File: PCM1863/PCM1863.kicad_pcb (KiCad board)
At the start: 2 copper layers, 76.2 x 128.5 mm, 64 parts, among them IC1 SN74AUC1G126DCKR, IC2 NCP163ASN330T1G, IC3 NCP163ASN330T1G, IC4 TXB0101DBVT, J1 Conn_02x05_Row_Letter_First, J10 Conn_01x10_Male, J4 USB_B_Micro, J8 Conn_01x10_Male, J9 Conn_01x10_Male, U1 PCM1863, Y1 ASE-24.000MHZ-ET, Y2 ASE-22.000MHZ-ET

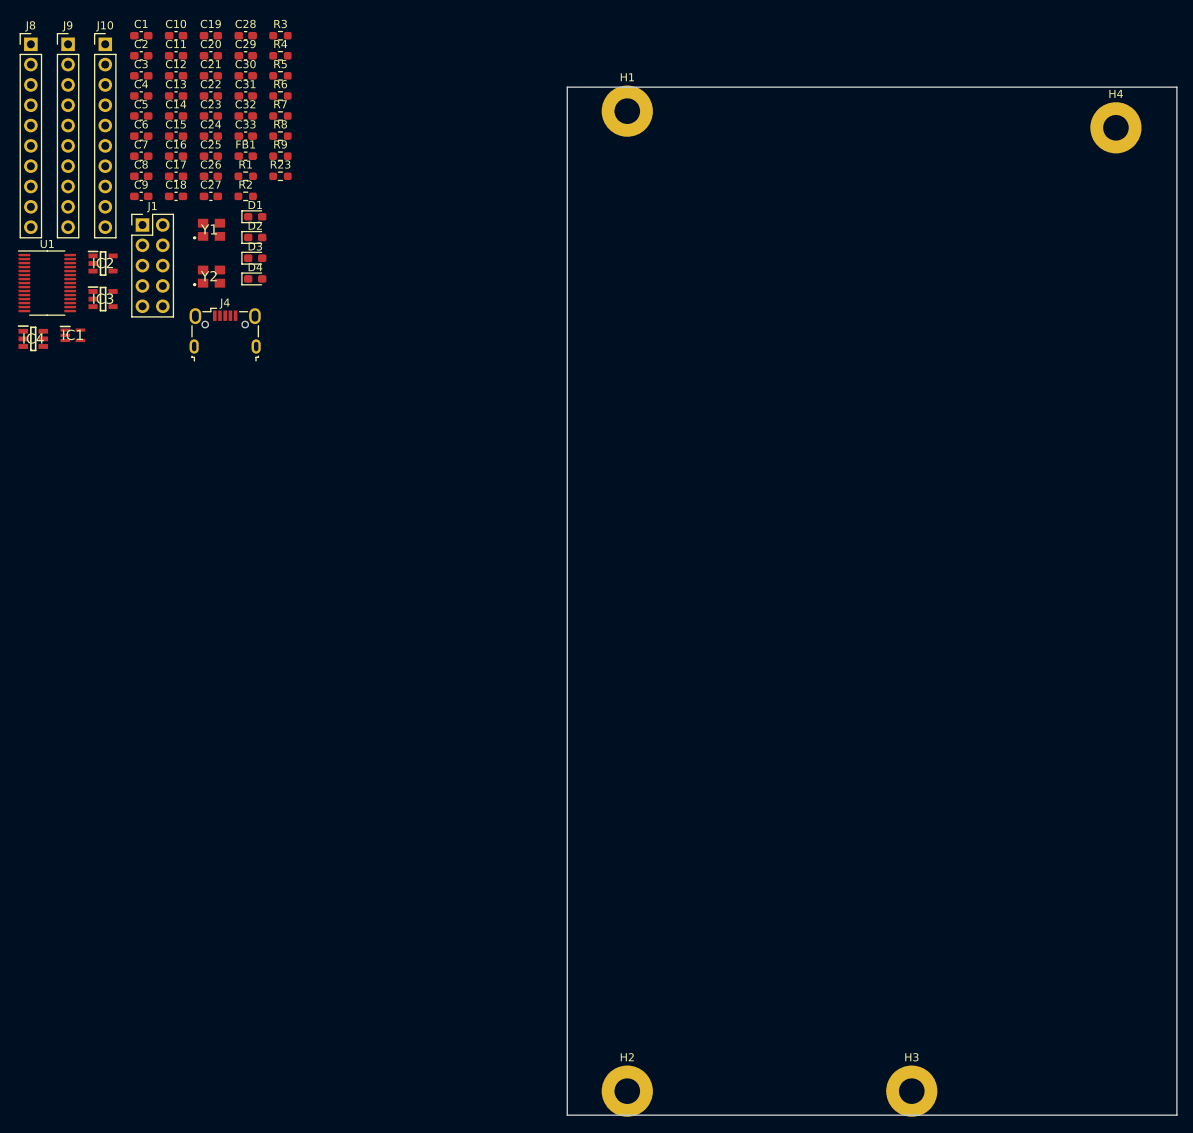
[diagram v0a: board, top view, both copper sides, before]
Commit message: Revert "Merge remote-tracking branch 'upstream/main'"
This reverts commit 91e618c32c18b3f8ce9c65181e2c7ed2aa69dacd, reversing
changes made to 5f9fe177db78953ec4a0d750e6893e90b3881885.
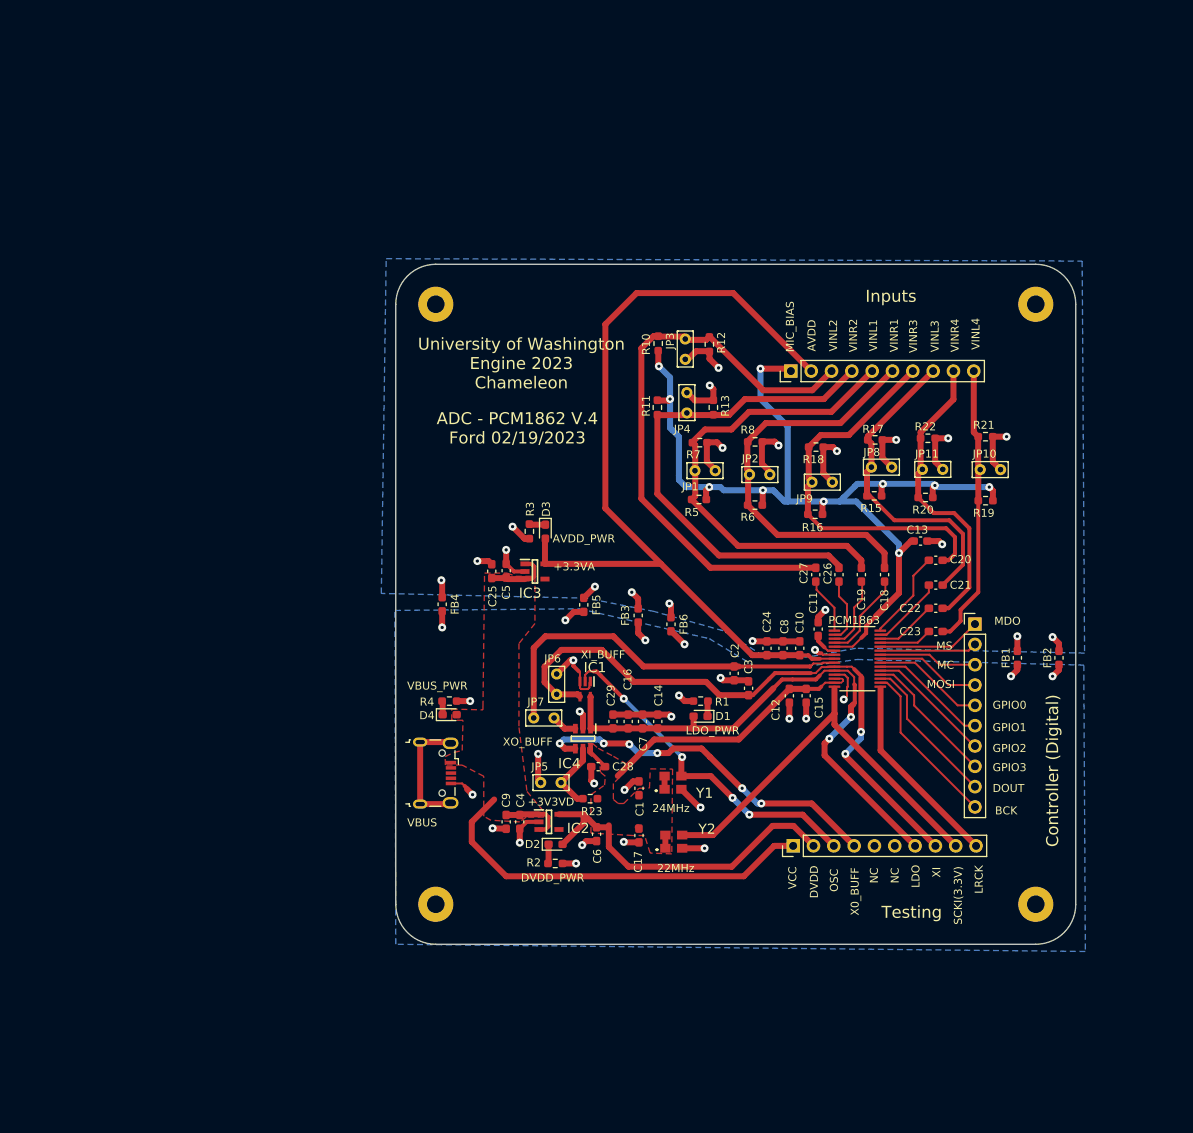
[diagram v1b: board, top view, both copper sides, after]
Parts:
- removed C30: 2.2uF, Capacitor_SMD:C_0603_1608Metric_Pad1.08x0.95mm_HandSolder
- removed C31, C33: 10uF, Capacitor_SMD:C_0603_1608Metric_Pad1.08x0.95mm_HandSolder
- removed C32: 0.01uF, Capacitor_SMD:C_0603_1608Metric_Pad1.08x0.95mm_HandSolder
- removed J10, J8, J9: Conn_01x10_Male, Connector_PinHeader_2.54mm:PinHeader_1x10_P2.54mm_Vertical
- removed R9: 4.99k, Resistor_SMD:R_0603_1608Metric_Pad0.98x0.95mm_HandSolder
- added FB2: FerriteBead, Inductor_SMD:L_0603_1608Metric_Pad1.05x0.95mm_HandSolder, F.Cu at (152.9, 94.2)
- added FB3: FerriteBead, Inductor_SMD:L_0603_1608Metric_Pad1.05x0.95mm_HandSolder, F.Cu at (100.3, 88.9)
- added FB4: FerriteBead, Inductor_SMD:L_0603_1608Metric_Pad1.05x0.95mm_HandSolder, F.Cu at (75.8, 87.5)
- added FB5: FerriteBead, Inductor_SMD:L_0603_1608Metric_Pad1.05x0.95mm_HandSolder, F.Cu at (93.5, 87.6)
- added FB6: FerriteBead, Inductor_SMD:L_0603_1608Metric_Pad1.05x0.95mm_HandSolder, F.Cu at (104.4, 90.0)
- added J2: Conn_01x10_Male, Connector_PinHeader_2.54mm:PinHeader_1x10_P2.54mm_Vertical, F.Cu at (119.4, 58.4)
- added J3: Conn_01x10_Male, Connector_PinHeader_2.54mm:PinHeader_1x10_P2.54mm_Vertical, F.Cu at (142.4, 90.0)
- added JP1: Jumper_2_Open, custom_lib:TestPoint_Bridge_Pitch2.54mm_Drill0.7mm, F.Cu at (106.2, 69.6)
- added JP10: Jumper_2_Open, custom_lib:TestPoint_Bridge_Pitch2.54mm_Drill0.7mm, F.Cu at (141.9, 69.5)
- added JP11: Jumper_2_Open, custom_lib:TestPoint_Bridge_Pitch2.54mm_Drill0.7mm, F.Cu at (139.6, 71.8)
- added JP2: Jumper_2_Open, custom_lib:TestPoint_Bridge_Pitch2.54mm_Drill0.7mm, F.Cu at (118.0, 72.5)
- added JP3: Jumper_2_Open, custom_lib:TestPoint_Bridge_Pitch2.54mm_Drill0.7mm, F.Cu at (107.4, 53.1)
- added JP4: Jumper_2_Open, custom_lib:TestPoint_Bridge_Pitch2.54mm_Drill0.7mm, F.Cu at (107.6, 59.8)
- added JP5: Jumper_2_Bridged, custom_lib:TestPoint_Bridge_Pitch2.54mm_Drill0.7mm, F.Cu at (91.9, 111.0)
- added JP6: Jumper_2_Open, custom_lib:TestPoint_Bridge_Pitch2.54mm_Drill0.7mm, F.Cu at (88.9, 100.0)
- added JP7: Jumper_2_Bridged, custom_lib:TestPoint_Bridge_Pitch2.54mm_Drill0.7mm, F.Cu at (86.0, 100.5)
- added JP8: Jumper_2_Open, custom_lib:TestPoint_Bridge_Pitch2.54mm_Drill0.7mm, F.Cu at (128.3, 69.2)
- added JP9: Jumper_2_Open, custom_lib:TestPoint_Bridge_Pitch2.54mm_Drill0.7mm, F.Cu at (125.8, 73.4)
- added R10: 2.2k, Resistor_SMD:R_0603_1608Metric_Pad0.98x0.95mm_HandSolder, F.Cu at (102.8, 54.9)
- added R11: 2.2k, Resistor_SMD:R_0603_1608Metric_Pad0.98x0.95mm_HandSolder, F.Cu at (102.7, 62.9)
- added R12: 100k, Resistor_SMD:R_0603_1608Metric_Pad0.98x0.95mm_HandSolder, F.Cu at (109.2, 55.0)
- added R13: 100k, Resistor_SMD:R_0603_1608Metric_Pad0.98x0.95mm_HandSolder, F.Cu at (109.7, 62.9)
- added R15: 2.2k, Resistor_SMD:R_0603_1608Metric_Pad0.98x0.95mm_HandSolder, F.Cu at (129.8, 74.0)
- added R16: 2.2k, Resistor_SMD:R_0603_1608Metric_Pad0.98x0.95mm_HandSolder, F.Cu at (122.4, 76.2)
- added R17: 100k, Resistor_SMD:R_0603_1608Metric_Pad0.98x0.95mm_HandSolder, F.Cu at (129.9, 67.0)
- added R18: 100k, Resistor_SMD:R_0603_1608Metric_Pad0.98x0.95mm_HandSolder, F.Cu at (122.5, 67.8)
- added R19: 2.2k, Resistor_SMD:R_0603_1608Metric_Pad0.98x0.95mm_HandSolder, F.Cu at (143.7, 74.5)
- added R20: 2.2k, Resistor_SMD:R_0603_1608Metric_Pad0.98x0.95mm_HandSolder, F.Cu at (136.2, 74.2)
- added R21: 100k, Resistor_SMD:R_0603_1608Metric_Pad0.98x0.95mm_HandSolder, F.Cu at (143.7, 66.5)
- added R22: 100k, Resistor_SMD:R_0603_1608Metric_Pad0.98x0.95mm_HandSolder, F.Cu at (136.5, 66.8)
- C10, C15, C16, C28, C29: value 0.1uF -> 0.1uF-16V
- C11: value 1uF -> 2.2uF
- C12, C14, C8: value 10uF-Tant -> 10uF-10V
- C13: value 0.1uF -> 0.1uF-50V
- C18, C19, C22: value 2.2uF -> 10uF-16V
- C2, C3: value 20pF -> 20pF-50V
- C20, C23, C27: value 0.01uF -> 10uF-16V
- C21, C26: value 10uF -> 10uF-16V
- C24: value 0.1uF -> 1uF
- C25, C9: value 10uF-Tant -> 10uF
- C5: value 1uF -> 0.1uF
- H1, H2, H3, H4: footprint MountingHole:MountingHole_3.2mm_M3_Pad -> MountingHole:MountingHole_2.2mm_M2_Pad
- J1: value Conn_02x05_Row_Letter_First -> Conn_01x10_Male; footprint Connector_PinHeader_2.54mm:PinHeader_2x05_P2.54mm_Vertical -> Connector_PinHeader_2.54mm:PinHeader_1x10_P2.54mm_Vertical
- R1, R5, R6: value 100 -> 2.2k
- R4: value 10k -> 2.2k
- R7, R8: value 100 -> 100k
- moved FB1 115.1 mm to (147.7, 94.2), turned to 90 degrees
- moved C1 112.8 mm to (100.4, 110.5), turned to 90 degrees
- moved J1 112.4 mm to (119.7, 117.7), turned to 90 degrees
- moved U1 111.6 mm to (127.7, 94.3)
- moved C23 111.2 mm to (137.5, 90.9), turned to 180 degrees
- moved C22 111.0 mm to (137.5, 88.0), turned to 180 degrees
- moved H2 110.8 mm to (150.0, 50.0)
- moved C21 110.7 mm to (137.5, 85.1), turned to 180 degrees
- moved C20 110.4 mm to (137.5, 82.0), turned to 180 degrees
- moved C10 109.3 mm to (120.5, 93.0), turned to -90 degrees
- moved C12 109.0 mm to (119.2, 98.9), turned to -90 degrees
- moved C13 108.4 mm to (135.6, 79.6), turned to 180 degrees
- moved C3 107.8 mm to (114.1, 98.0), turned to -90 degrees
- moved C11 107.6 mm to (122.8, 90.6), turned to -90 degrees
- moved C2 107.0 mm to (112.3, 96.1), turned to 90 degrees
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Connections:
- net /XO_EN renamed Net-(IC4-Pad5)
- net Net-(U1-VINR4/VIN3M) renamed /4R
- C1 pad 1: +3V3 -> DVDD
- C10 pad 2: +3.3VA -> AVDD
- C11 pad 2: /VREF_gnd -> Net-(C11-Pad2)
- C12 pad 1: +3V3 -> DVDD
- C13 pad 2: Net-(U1-Mic_Bias) -> MICBIAS
- C14 pad 1: +1V8 -> LDO
- C15 pad 1: +3V3 -> DVDD
- C16 pad 1: +1V8 -> LDO
- C17 pad 1: +3V3 -> DVDD
- C18 pad 1: GNDA -> VINR1
- C18 pad 2: Net-(U1-VINR2/VIN2M) -> /1R
- C19 pad 1: GNDA -> VINL1
- C19 pad 2: Net-(U1-VINL2/VIN1M) -> /1L
- C2 pad 1: /XO_gnd -> GNDD
- C2 pad 2: GNDD -> XO
- C20 pad 1: GNDA -> VINR3
- C20 pad 2: /VIN4P -> /3R
- C21 pad 1: Net-(C21-Pad1) -> VINL3
- C21 pad 2: /IN4 -> /3L
- C22 pad 1: GNDA -> VINR4
- C23 pad 1: GNDA -> VINL4
- C23 pad 2: /VIN3P -> /4L
- C24 pad 1: VCC -> GNDA
- C24 pad 2: GNDA -> AVDD
- C26 pad 1: Net-(C26-Pad1) -> VINR2
- C26 pad 2: /IN3 -> /2R
- C27 pad 1: GNDA -> VINL2
- C27 pad 2: /VIN2P -> /2L
- C28 pad 1: +3V3 -> DVDD
- C29 pad 2: +1V8 -> LDO
- C3 pad 2: /XI_gnd -> XI
- C5 pad 1: GNDA -> VCC
- C5 pad 2: +3.3VA -> GNDA
- C6 pad 2: +3V3 -> DVDD
- C7 pad 1: +1V8 -> LDO
- C8 pad 2: +3.3VA -> AVDD
- D1 pad 2: +1V8 -> LDO
- D2 pad 2: +3V3 -> DVDD
- D3 pad 2: +3.3VA -> AVDD
- H1 pad 1: GNDD -> GNDA
- H3 pad 1: GNDA -> GNDD
- IC1 pad 1: /XI_EN -> GNDD
- IC1 pad 2: /OSC -> OSC
- IC1 pad 4: /XI -> XI
- IC1 pad 5: +1V8 -> LDO
- IC2 pad 5: +3V3 -> DVDD
- IC3 pad 5: +3.3VA -> AVDD
- IC4 pad 1: +1V8 -> LDO
- IC4 pad 3: /XO -> Net-(IC4-Pad3)
- IC4 pad 4: /XO_BUFF -> XO_BUFF
- IC4 pad 6: +3V3 -> DVDD
- J1 pad 1: (no net) -> VCC
- J1 pad 10: (no net) -> LRCK
- J1 pad 2: (no net) -> DVDD
- J1 pad 3: (no net) -> OSC
- J1 pad 4: (no net) -> XO_BUFF
- J1 pad 5: (no net) -> unconnected-(J1-Pad5)
- J1 pad 6: (no net) -> unconnected-(J1-Pad6)
- J1 pad 7: (no net) -> LDO
- J1 pad 8: (no net) -> XI
- J1 pad 9: (no net) -> SCKI(3.3V)
- J4 pad 6: GNDD -> unconnected-(J4-Pad6)
- R23 pad 1: +3V3 -> DVDD
- R5 pad 1: Net-(C21-Pad1) -> MICBIAS
- R5 pad 2: /VIN4P -> VINL1
- R6 pad 1: Net-(C26-Pad1) -> MICBIAS
- R6 pad 2: /VIN3P -> VINR1
- R7 pad 1: Net-(C31-Pad1) -> GNDA
- R7 pad 2: /VIN2P -> VINL1
- R8 pad 1: Net-(C33-Pad1) -> VINR1
- R8 pad 2: /VIN1P -> GNDA
- U1 pad 1: Net-(U1-VINL2/VIN1M) -> /2L
- U1 pad 10: /XI -> XI
- U1 pad 11: +1V8 -> LDO
- U1 pad 13: +3V3 -> DVDD
- U1 pad 14: +3V3 -> DVDD
- U1 pad 15: /SCKI(3.3V) -> SCKI(3.3V)
- U1 pad 16: /LRCK -> LRCK
- U1 pad 17: /BCK -> BCK
- U1 pad 18: /DOUT -> DOUT
- U1 pad 2: Net-(U1-VINR2/VIN2M) -> /2R
- U1 pad 27: Net-(U1-VINL4/VIN4M) -> /4L
- U1 pad 29: /VIN4P -> /3L
- U1 pad 3: /VIN1P -> /1L
- U1 pad 30: /VIN3P -> /3R
- U1 pad 4: /VIN2P -> /1R
- U1 pad 5: Net-(U1-Mic_Bias) -> MICBIAS
- U1 pad 6: /VREF -> Net-(C11-Pad2)
- U1 pad 8: +3.3VA -> AVDD
- U1 pad 9: /XO -> XO
- Y1 pad 1: +3V3 -> DVDD
- Y1 pad 3: /SCKI(3.3V) -> OSC
- Y1 pad 4: +3V3 -> DVDD
- Y2 pad 1: +3V3 -> DVDD
- Y2 pad 3: /OSC -> SCKI(3.3V)
- Y2 pad 4: +3V3 -> DVDD
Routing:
- net MICBIAS: track 0.00 -> 121.5 mm, vias 0 -> 10
- net AVDD: track 0.00 -> 108.4 mm
- net DVDD: track 0.00 -> 84.8 mm
- net GNDA: track 0.00 -> 83.2 mm, vias 0 -> 21
- net XI: track 0.00 -> 78.6 mm, vias 0 -> 2
- net GNDD: track 0.00 -> 77.2 mm, vias 0 -> 26
- net VINL2: track 0.00 -> 72.7 mm
- net LDO: track 0.00 -> 69.2 mm, vias 0 -> 2
- net VCC: track 0.00 -> 66.1 mm
- net VINR2: track 0.00 -> 63.4 mm
- net VINL1: track 0.00 -> 59.0 mm
- net VINR1: track 0.00 -> 51.4 mm
- net SCKI(3.3V): track 0.00 -> 51.3 mm
- net XO: track 0.00 -> 49.3 mm
- net VINR3: track 0.00 -> 49.3 mm
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- added copper zone on F.Cu, net DVDD
- added copper zone on B.Cu, net GNDA
- added copper zone on B.Cu, net GNDD
- added copper zone on F.Cu, net VCC
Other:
- board size 76.2 x 128.5 mm -> 85 x 85 mm
- board text added: "+3.3VA"
- board text added: "+3V3VD"
- board text added: "22MHz"
- board text added: "24MHz"
- board text added: "ADC - PCM1862 V.4 Ford 02/19/2023"
- board text added: "AVDD"
- board text added: "AVDD_PWR"
- board text added: "BCK"
- board text added: "Controller (Digital)"
- board text added: "DOUT"
- board text added: "DVDD"
- board text added: "DVDD_PWR"
- board text added: "GPIO0"
- board text added: "GPIO1"
- board text added: "GPIO2"
- board text added: "GPIO3"
- board text added: "Inputs"
- board text added: "LDO"
- board text added: "LDO_PWR"
- board text added: "LRCK"
- board text added: "MC"
- board text added: "MDO"
- board text added: "MIC_BIAS"
- board text added: "MOSI"
- board text added: "MS"
- board text added: "NC"
- board text added: "OSC"
- board text added: "PCM1863"
- board text added: "SCKI(3.3V)"
- board text added: "Testing"
- board text added: "University of Washington Engine 2023 Chameleon"
- board text added: "VBUS"
- board text added: "VBUS_PWR"
- board text added: "VCC"
- board text added: "VINL1"
- board text added: "VINL2"
- board text added: "VINL3"
- board text added: "VINL4"
- board text added: "VINR1"
- board text added: "VINR2"
- board text added: "VINR3"
- board text added: "VINR4"
- board text added: "X0_BUFF"
- board text added: "XI"
- board text added: "XI_BUFF"
- board text added: "XO_BUFF"

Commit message: Revert "Revert "Merge remote-tracking branch 'upstream/main'""
This reverts commit 1d57ca07421005fad3c6f783a10b39dbb3c17bbf.
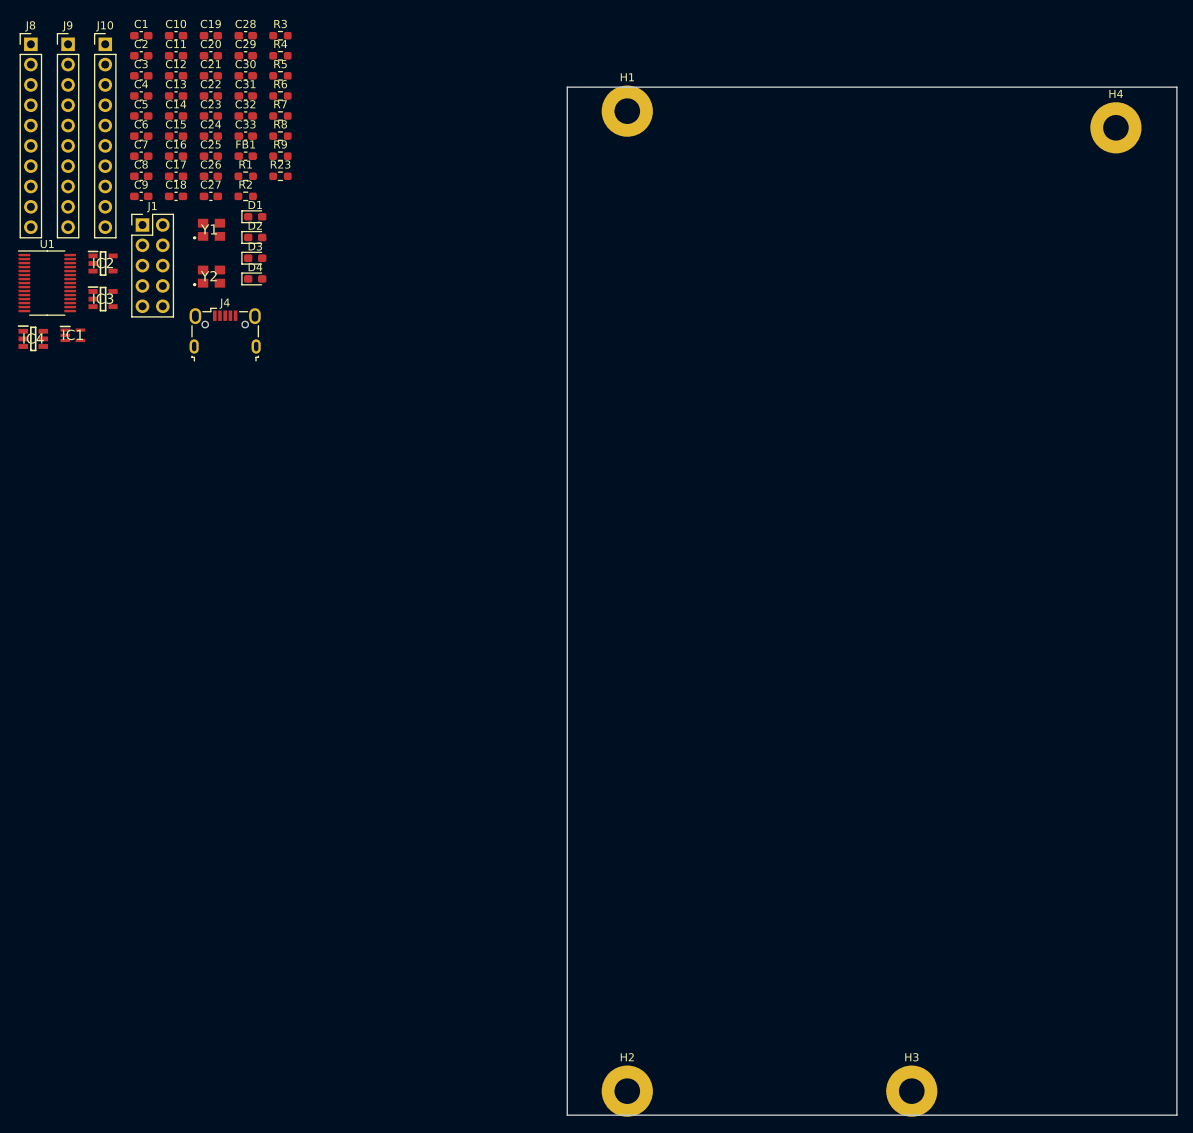
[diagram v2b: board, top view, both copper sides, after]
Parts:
- removed FB2, FB3, FB4, FB5, FB6: FerriteBead, Inductor_SMD:L_0603_1608Metric_Pad1.05x0.95mm_HandSolder
- removed J2, J3: Conn_01x10_Male, Connector_PinHeader_2.54mm:PinHeader_1x10_P2.54mm_Vertical
- removed JP1, JP10, JP11, JP2, JP3, JP4, JP6, JP8, JP9: Jumper_2_Open, custom_lib:TestPoint_Bridge_Pitch2.54mm_Drill0.7mm
- removed JP5, JP7: Jumper_2_Bridged, custom_lib:TestPoint_Bridge_Pitch2.54mm_Drill0.7mm
- removed R10, R11, R15, R16, R19, R20: 2.2k, Resistor_SMD:R_0603_1608Metric_Pad0.98x0.95mm_HandSolder
- removed R12, R13, R17, R18, R21, R22: 100k, Resistor_SMD:R_0603_1608Metric_Pad0.98x0.95mm_HandSolder
- added C30: 2.2uF, Capacitor_SMD:C_0603_1608Metric_Pad1.08x0.95mm_HandSolder, F.Cu at (51.2, 21.4)
- added C31: 10uF, Capacitor_SMD:C_0603_1608Metric_Pad1.08x0.95mm_HandSolder, F.Cu at (51.2, 24.0)
- added C32: 0.01uF, Capacitor_SMD:C_0603_1608Metric_Pad1.08x0.95mm_HandSolder, F.Cu at (51.2, 26.5)
- added C33: 10uF, Capacitor_SMD:C_0603_1608Metric_Pad1.08x0.95mm_HandSolder, F.Cu at (51.2, 29.0)
- added J10: Conn_01x10_Male, Connector_PinHeader_2.54mm:PinHeader_1x10_P2.54mm_Vertical, F.Cu at (33.7, 17.5)
- added J8: Conn_01x10_Male, Connector_PinHeader_2.54mm:PinHeader_1x10_P2.54mm_Vertical, F.Cu at (24.4, 17.5)
- added J9: Conn_01x10_Male, Connector_PinHeader_2.54mm:PinHeader_1x10_P2.54mm_Vertical, F.Cu at (29.0, 17.5)
- added R9: 4.99k, Resistor_SMD:R_0603_1608Metric_Pad0.98x0.95mm_HandSolder, F.Cu at (55.6, 31.5)
- C10, C15, C16, C28, C29: value 0.1uF-16V -> 0.1uF
- C11: value 2.2uF -> 1uF
- C12, C14, C8: value 10uF-10V -> 10uF-Tant
- C13: value 0.1uF-50V -> 0.1uF
- C18, C19, C22: value 10uF-16V -> 2.2uF
- C2, C3: value 20pF-50V -> 20pF
- C20, C23, C27: value 10uF-16V -> 0.01uF
- C21, C26: value 10uF-16V -> 10uF
- C24: value 1uF -> 0.1uF
- C25, C9: value 10uF -> 10uF-Tant
- C5: value 0.1uF -> 1uF
- H1, H2, H3, H4: footprint MountingHole:MountingHole_2.2mm_M2_Pad -> MountingHole:MountingHole_3.2mm_M3_Pad
- J1: value Conn_01x10_Male -> Conn_02x05_Row_Letter_First; footprint Connector_PinHeader_2.54mm:PinHeader_1x10_P2.54mm_Vertical -> Connector_PinHeader_2.54mm:PinHeader_2x05_P2.54mm_Vertical
- R1, R5, R6: value 2.2k -> 100
- R4: value 2.2k -> 10k
- R7, R8: value 100k -> 100
- moved FB1 115.1 mm to (51.2, 31.5), turned to 0 degrees
- moved C1 112.8 mm to (38.2, 16.4), turned to 0 degrees
- moved J1 112.4 mm to (38.3, 40.1), turned to 0 degrees
- moved U1 111.6 mm to (26.4, 47.4)
- moved C23 111.2 mm to (46.9, 26.5), turned to 0 degrees
- moved C22 111.0 mm to (46.9, 24.0), turned to 0 degrees
- moved H2 110.8 mm to (98.9, 148.4)
- moved C21 110.7 mm to (46.9, 21.4), turned to 0 degrees
- moved C20 110.4 mm to (46.9, 18.9), turned to 0 degrees
- moved C10 109.3 mm to (42.5, 16.4), turned to 0 degrees
- moved C12 109.0 mm to (42.5, 21.4), turned to 0 degrees
- moved C13 108.4 mm to (42.5, 24.0), turned to 0 degrees
- moved C3 107.8 mm to (38.2, 21.4), turned to 0 degrees
- moved C11 107.6 mm to (42.5, 18.9), turned to 0 degrees
- moved C2 107.0 mm to (38.2, 18.9), turned to 0 degrees
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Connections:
- net /4R renamed Net-(U1-VINR4/VIN3M)
- net Net-(IC4-Pad5) renamed /XO_EN
- C1 pad 1: DVDD -> +3V3
- C10 pad 2: AVDD -> +3.3VA
- C11 pad 2: Net-(C11-Pad2) -> /VREF_gnd
- C12 pad 1: DVDD -> +3V3
- C13 pad 2: MICBIAS -> Net-(U1-Mic_Bias)
- C14 pad 1: LDO -> +1V8
- C15 pad 1: DVDD -> +3V3
- C16 pad 1: LDO -> +1V8
- C17 pad 1: DVDD -> +3V3
- C18 pad 1: VINR1 -> GNDA
- C18 pad 2: /1R -> Net-(U1-VINR2/VIN2M)
- C19 pad 1: VINL1 -> GNDA
- C19 pad 2: /1L -> Net-(U1-VINL2/VIN1M)
- C2 pad 1: GNDD -> /XO_gnd
- C2 pad 2: XO -> GNDD
- C20 pad 1: VINR3 -> GNDA
- C20 pad 2: /3R -> /VIN4P
- C21 pad 1: VINL3 -> Net-(C21-Pad1)
- C21 pad 2: /3L -> /IN4
- C22 pad 1: VINR4 -> GNDA
- C23 pad 1: VINL4 -> GNDA
- C23 pad 2: /4L -> /VIN3P
- C24 pad 1: GNDA -> VCC
- C24 pad 2: AVDD -> GNDA
- C26 pad 1: VINR2 -> Net-(C26-Pad1)
- C26 pad 2: /2R -> /IN3
- C27 pad 1: VINL2 -> GNDA
- C27 pad 2: /2L -> /VIN2P
- C28 pad 1: DVDD -> +3V3
- C29 pad 2: LDO -> +1V8
- C3 pad 2: XI -> /XI_gnd
- C5 pad 1: VCC -> GNDA
- C5 pad 2: GNDA -> +3.3VA
- C6 pad 2: DVDD -> +3V3
- C7 pad 1: LDO -> +1V8
- C8 pad 2: AVDD -> +3.3VA
- D1 pad 2: LDO -> +1V8
- D2 pad 2: DVDD -> +3V3
- D3 pad 2: AVDD -> +3.3VA
- H1 pad 1: GNDA -> GNDD
- H3 pad 1: GNDD -> GNDA
- IC1 pad 1: GNDD -> /XI_EN
- IC1 pad 2: OSC -> /OSC
- IC1 pad 4: XI -> /XI
- IC1 pad 5: LDO -> +1V8
- IC2 pad 5: DVDD -> +3V3
- IC3 pad 5: AVDD -> +3.3VA
- IC4 pad 1: LDO -> +1V8
- IC4 pad 3: Net-(IC4-Pad3) -> /XO
- IC4 pad 4: XO_BUFF -> /XO_BUFF
- IC4 pad 6: DVDD -> +3V3
- J1 pad 1: VCC -> (no net)
- J1 pad 10: LRCK -> (no net)
- J1 pad 2: DVDD -> (no net)
- J1 pad 3: OSC -> (no net)
- J1 pad 4: XO_BUFF -> (no net)
- J1 pad 5: unconnected-(J1-Pad5) -> (no net)
- J1 pad 6: unconnected-(J1-Pad6) -> (no net)
- J1 pad 7: LDO -> (no net)
- J1 pad 8: XI -> (no net)
- J1 pad 9: SCKI(3.3V) -> (no net)
- J4 pad 6: unconnected-(J4-Pad6) -> GNDD
- R23 pad 1: DVDD -> +3V3
- R5 pad 1: MICBIAS -> Net-(C21-Pad1)
- R5 pad 2: VINL1 -> /VIN4P
- R6 pad 1: MICBIAS -> Net-(C26-Pad1)
- R6 pad 2: VINR1 -> /VIN3P
- R7 pad 1: GNDA -> Net-(C31-Pad1)
- R7 pad 2: VINL1 -> /VIN2P
- R8 pad 1: VINR1 -> Net-(C33-Pad1)
- R8 pad 2: GNDA -> /VIN1P
- U1 pad 1: /2L -> Net-(U1-VINL2/VIN1M)
- U1 pad 10: XI -> /XI
- U1 pad 11: LDO -> +1V8
- U1 pad 13: DVDD -> +3V3
- U1 pad 14: DVDD -> +3V3
- U1 pad 15: SCKI(3.3V) -> /SCKI(3.3V)
- U1 pad 16: LRCK -> /LRCK
- U1 pad 17: BCK -> /BCK
- U1 pad 18: DOUT -> /DOUT
- U1 pad 2: /2R -> Net-(U1-VINR2/VIN2M)
- U1 pad 27: /4L -> Net-(U1-VINL4/VIN4M)
- U1 pad 29: /3L -> /VIN4P
- U1 pad 3: /1L -> /VIN1P
- U1 pad 30: /3R -> /VIN3P
- U1 pad 4: /1R -> /VIN2P
- U1 pad 5: MICBIAS -> Net-(U1-Mic_Bias)
- U1 pad 6: Net-(C11-Pad2) -> /VREF
- U1 pad 8: AVDD -> +3.3VA
- U1 pad 9: XO -> /XO
- Y1 pad 1: DVDD -> +3V3
- Y1 pad 3: OSC -> /SCKI(3.3V)
- Y1 pad 4: DVDD -> +3V3
- Y2 pad 1: DVDD -> +3V3
- Y2 pad 3: SCKI(3.3V) -> /OSC
- Y2 pad 4: DVDD -> +3V3
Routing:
- net MICBIAS: track 121.5 -> 0.00 mm, vias 10 -> 0
- net AVDD: track 108.4 -> 0.00 mm
- net DVDD: track 84.8 -> 0.00 mm
- net GNDA: track 83.2 -> 0.00 mm, vias 21 -> 0
- net XI: track 78.6 -> 0.00 mm, vias 2 -> 0
- net GNDD: track 77.2 -> 0.00 mm, vias 26 -> 0
- net VINL2: track 72.7 -> 0.00 mm
- net LDO: track 69.2 -> 0.00 mm, vias 2 -> 0
- net VCC: track 66.1 -> 0.00 mm
- net VINR2: track 63.4 -> 0.00 mm
- net VINL1: track 59.0 -> 0.00 mm
- net VINR1: track 51.4 -> 0.00 mm
- net SCKI(3.3V): track 51.3 -> 0.00 mm
- net XO: track 49.3 -> 0.00 mm
- net VINR3: track 49.3 -> 0.00 mm
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- removed copper zone on F.Cu, net DVDD
- removed copper zone on B.Cu, net GNDA
- removed copper zone on B.Cu, net GNDD
- removed copper zone on F.Cu, net VCC
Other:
- board size 85 x 85 mm -> 76.2 x 128.5 mm
- board text removed: "+3.3VA"
- board text removed: "+3V3VD"
- board text removed: "22MHz"
- board text removed: "24MHz"
- board text removed: "ADC - PCM1862 V.4 Ford 02/19/2023"
- board text removed: "AVDD"
- board text removed: "AVDD_PWR"
- board text removed: "BCK"
- board text removed: "Controller (Digital)"
- board text removed: "DOUT"
- board text removed: "DVDD"
- board text removed: "DVDD_PWR"
- board text removed: "GPIO0"
- board text removed: "GPIO1"
- board text removed: "GPIO2"
- board text removed: "GPIO3"
- board text removed: "Inputs"
- board text removed: "LDO"
- board text removed: "LDO_PWR"
- board text removed: "LRCK"
- board text removed: "MC"
- board text removed: "MDO"
- board text removed: "MIC_BIAS"
- board text removed: "MOSI"
- board text removed: "MS"
- board text removed: "NC"
- board text removed: "OSC"
- board text removed: "PCM1863"
- board text removed: "SCKI(3.3V)"
- board text removed: "Testing"
- board text removed: "University of Washington Engine 2023 Chameleon"
- board text removed: "VBUS"
- board text removed: "VBUS_PWR"
- board text removed: "VCC"
- board text removed: "VINL1"
- board text removed: "VINL2"
- board text removed: "VINL3"
- board text removed: "VINL4"
- board text removed: "VINR1"
- board text removed: "VINR2"
- board text removed: "VINR3"
- board text removed: "VINR4"
- board text removed: "X0_BUFF"
- board text removed: "XI"
- board text removed: "XI_BUFF"
- board text removed: "XO_BUFF"
